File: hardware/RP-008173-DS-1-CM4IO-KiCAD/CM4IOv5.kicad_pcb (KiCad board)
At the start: 4 copper layers, 160 x 90 mm, 151 parts, among them J1 Conn_01x03, J10 690-019-298-412, J11 USB_OTG, J12 10018783-11200TLF, J13 690-008-221-904, J14 Conn_02x05_Odd_Even, J15 Conn_01x22_Female, J16 Conn_01x22_Female, J17 Molex 470531000, J19 Barrel_Jack, J2 Conn_02x07_Odd_Even, J20 AMP171826-4, J22 690-019-298-412, J3 Conn_01x03, J4 Conn_01x22_Female, J5 Conn_01x22_Female, J6 THD-02-R, J7 Micro_SD_Card_Det, J8 THD-20-R, J9 THD-02-R, Q1 DMP3013SFV-7, U1 TPD4EUSB30, U11 EMC2301-1-ACZL-TR, U12 RT9742SNGV, U13 FSUSB42MUX, U14 74LVC1G07SE-7, U15 AP64501SP-13, U16 AP64501SP-13, U18 RT9742GGJ5, U2 TPD4EUSB30, U3 MagJack-A70-112-331N126, U4 TPD4EUSB30, U5 74LVC1G07SE-7, U6 USB2514B-I/M2, U7 AP22653W6, U8 PCF85063AT/AAZ, U9 74LVC1G07SE-7, Y1 24MHz, Y2 X32K768S301

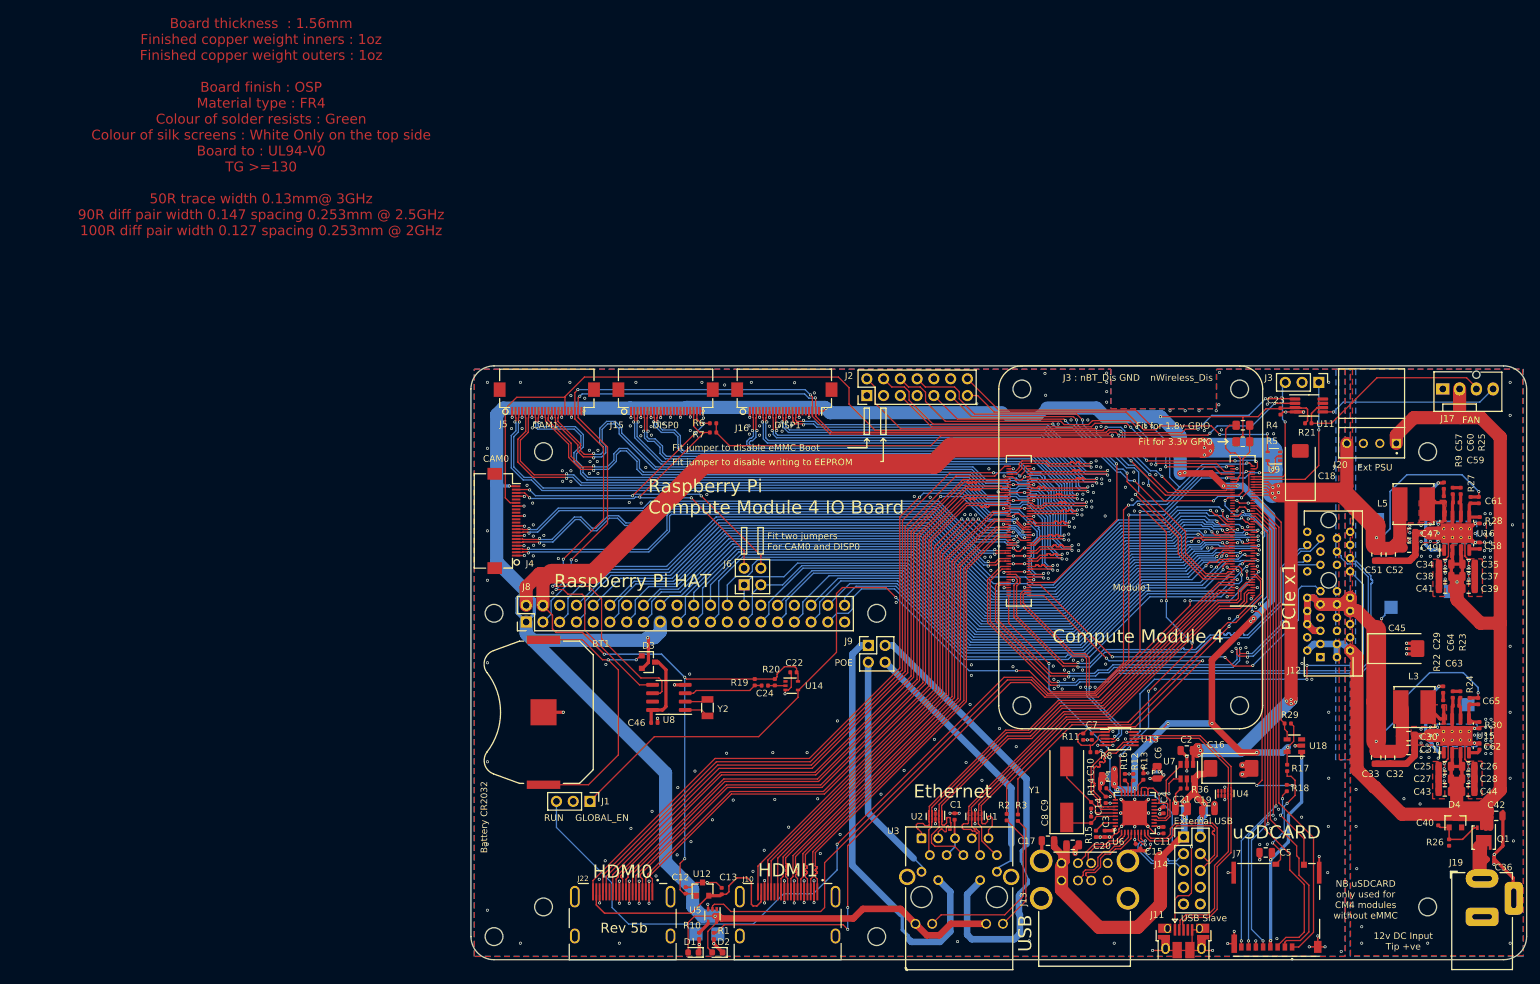
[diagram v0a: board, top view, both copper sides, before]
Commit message: added current project
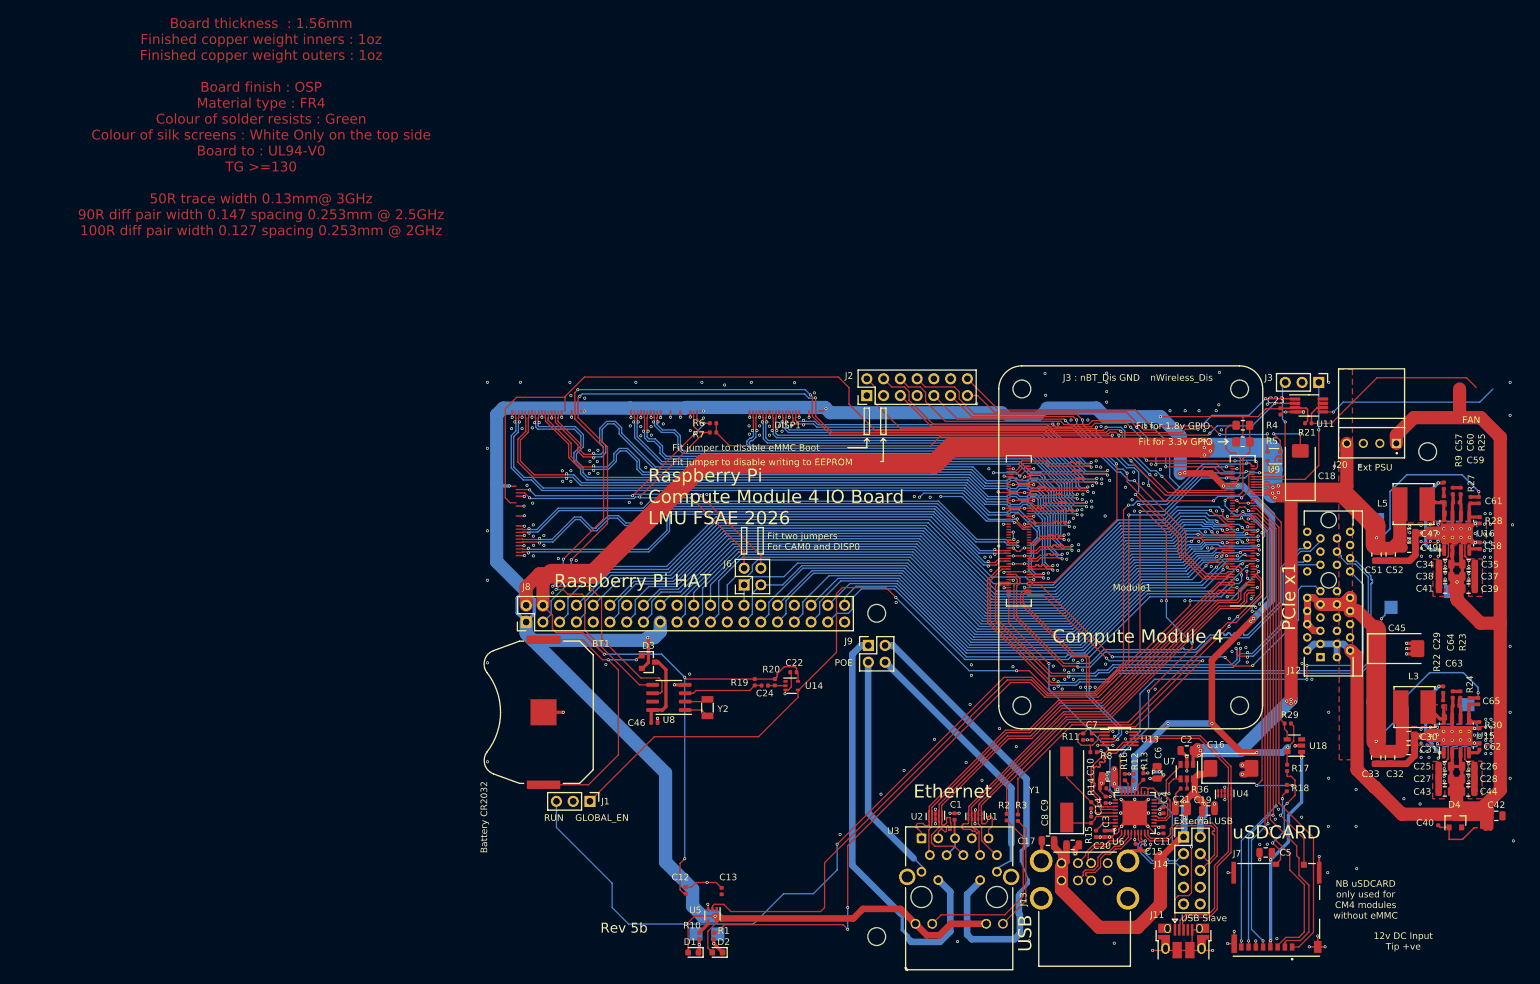
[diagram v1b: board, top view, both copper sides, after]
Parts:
- removed C36: 100n 100v, Capacitor_SMD:C_0402_1005Metric
- removed H1, H2, H3, H7, H8: MountingHole, MountingHole:MountingHole_2.7mm_M2.5
- removed J10, J22: 690-019-298-412, CM4IO:EDAC 690-019-298-412
- removed J15, J16, J4, J5: Conn_01x22_Female, CM4IO:Hirose_FH12-22S-0.5SH_1x22-1MP_P0.50mm_Horizontal
- removed J17: Molex 470531000, Connector:FanPinHeader_1x04_P2.54mm_Vertical
- removed J19: Barrel_Jack, CM4IO:BarrelJack_Horizontal
- removed Q1: DMP3013SFV-7, Package_SON:Diodes_PowerDI3333-8
- removed R26: 12K 1%, Resistor_SMD:R_0402_1005Metric
- removed U12: RT9742SNGV, Package_TO_SOT_SMD:SOT-23
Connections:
- net /CM4_HighSpeed/SCL0 renamed /RTC , Wakeup, FAN/SCL
- net /CM4_HighSpeed/SDA0 renamed /RTC , Wakeup, FAN/SDA
- C34 pad 1: /+12v -> /PSUs/+12v
- C35 pad 1: /+12v -> /PSUs/+12v
- C37 pad 1: /+12v -> /PSUs/+12v
- C38 pad 1: /+12v -> /PSUs/+12v
- C39 pad 1: /+12v -> /PSUs/+12v
- C41 pad 1: /+12v -> /PSUs/+12v
- Module1 pad 97: /CM4_HighSpeed/CAM_GPIO -> /CM4_GPIO ( Ethernet, GPIO, SDCARD)/CAM_GPIO
- U16 pad 2: /+12v -> /PSUs/+12v
- U16 pad 3: /+12v -> /PSUs/+12v
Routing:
- net /CM4_HighSpeed/CAM_GPIO: track 143.1 -> 0.00 mm, vias 4 -> 0
- net /CM4_GPIO ( Ethernet, GPIO, SDCARD)/CAM_GPIO: track 0.00 -> 143.1 mm, vias 0 -> 4
- net /CM4_HighSpeed/HDMI0_SCL: track 101.9 -> 0.00 mm
- net /CM4_HighSpeed/HDMI0_SDA: track 106.8 -> 6.56 mm
- net /CM4_HighSpeed/HDMI0_CK_P: track 99.6 -> 0.00 mm
- net /CM4_HighSpeed/HDMI0_CK_N: track 99.6 -> 0.00 mm
- net /CM4_HighSpeed/HDMI0_D0_N: track 98.2 -> 0.00 mm
- net /CM4_HighSpeed/HDMI0_D0_P: track 98.2 -> 0.00 mm
- net /CM4_HighSpeed/HDMI0_D1_P: track 95.8 -> 0.00 mm
- net /CM4_HighSpeed/HDMI0_D1_N: track 95.7 -> 0.00 mm
- net /CM4_HighSpeed/HDMI0_D2_N: track 93.8 -> 0.00 mm
- net /CM4_HighSpeed/HDMI0_D2_P: track 93.7 -> 0.00 mm
- net /CM4_HighSpeed/HDMI0_CEC: track 104.2 -> 15.4 mm
- net /CM4_HighSpeed/HDMI0_HOTPLUG: track 108.0 -> 19.3 mm
- net /CM4_HighSpeed/HDMI1_HOTPLUG: track 80.8 -> 0.00 mm, vias 2 -> 0
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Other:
- board outline removed
- board text added: "Raspberry Pi Compute Module 4 IO Board LMU FSAE 2026"
- board text removed: "CAM0"
- board text removed: "CAM1"
- board text removed: "DISP0"
- board text removed: "HDMI0"
- board text removed: "HDMI1"
- board text removed: "Raspberry Pi Compute Module 4 IO Board"
